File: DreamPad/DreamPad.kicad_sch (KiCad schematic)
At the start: 25 parts, among them J1 OLED Display, SW1 SW_Push, SW10 SW_Push, SW11 SW_Push, SW13 RotaryEncoder_Switch, SW2 SW_Push, SW3 SW_Push, SW5 SW_Push, SW6 SW_Push, SW7 SW_Push, SW9 SW_Push, U1 MOUDLE-SEEEDUINO-XIAO

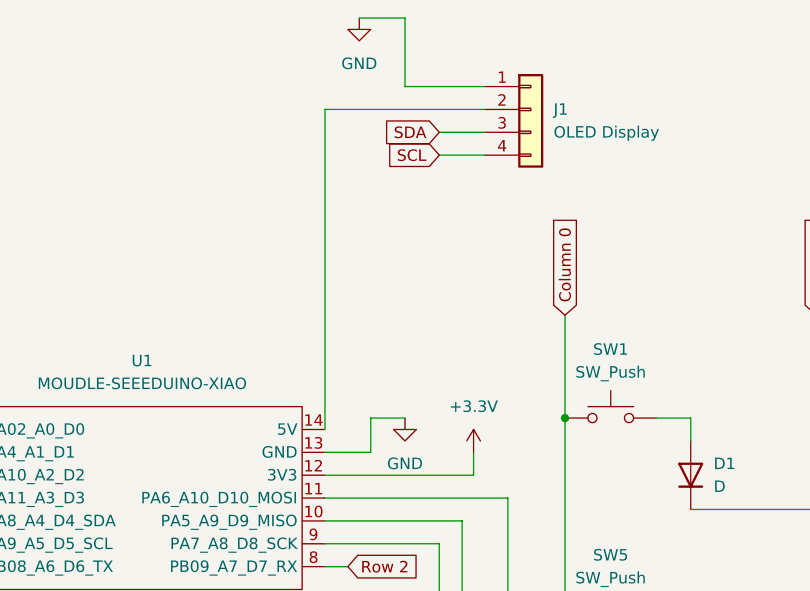
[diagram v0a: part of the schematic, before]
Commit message: Finalization and Readme
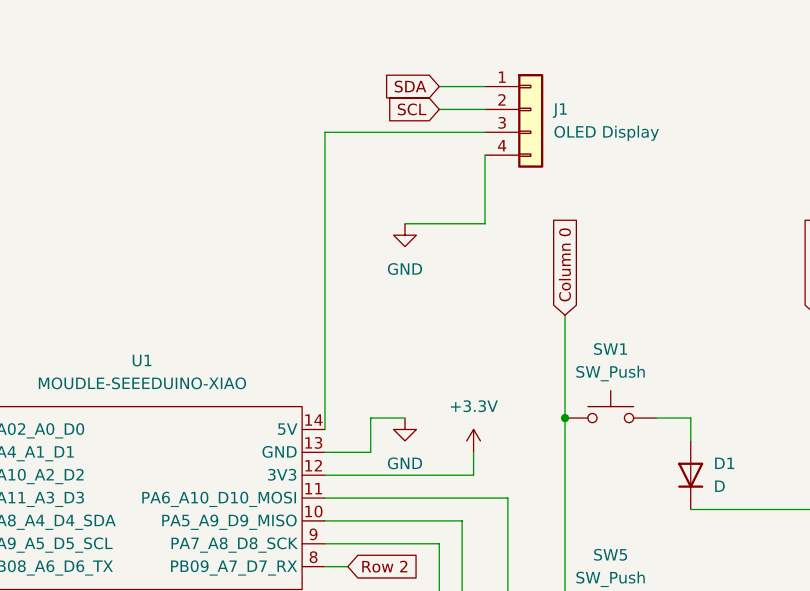
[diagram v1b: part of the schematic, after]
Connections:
- net GND: now also J1.4 (Pin_4); no longer J1.1 (Pin_1)
- net SCL: now also J1.2 (Pin_2); no longer J1.4 (Pin_4)
- net SDA: now also J1.1 (Pin_1); no longer J1.3 (Pin_3)
- net at U1.14 (5V): now also J1.3 (Pin_3); no longer J1.2 (Pin_2)
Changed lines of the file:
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@@
+	(wire
+		(pts
+			(xy 156.21 41.91) (xy 156.21 34.29)
+		)
+		(stroke
+			(width 0)
+			(type default)
+		)
+	)
 	(wire
 		(pts
@@
 	(wire
 		(pts
-			(xy 151.13 34.29) (xy 156.21 34.29)
-		)
-		(stroke
-			(width 0)
-			(type default)
-		)
-	)
-	(wire
-		(pts
-			(xy 142.24 19.05) (xy 147.32 19.05)
+			(xy 138.43 64.77) (xy 138.43 31.75)
 		)
 		(stroke
@@
 	(wire
 		(pts
-			(xy 138.43 29.21) (xy 138.43 64.77)
-		)
-		(stroke
-			(width 0)
-			(type default)
-		)
-	)
-	(wire
-		(pts
 			(xy 179.07 109.22) (xy 179.07 111.76)
 		)
@@
 	(wire
 		(pts
-			(xy 156.21 26.67) (xy 147.32 26.67)
-		)
-		(stroke
-			(width 0)
-			(type default)
-		)
-	)
-	(wire
-		(pts
 			(xy 88.9 69.85) (xy 97.79 69.85)
 		)
@@
 	(wire
 		(pts
+			(xy 151.13 29.21) (xy 156.21 29.21)
+		)
+		(stroke
+			(width 0)
+			(type default)
+		)
+	)
+	(wire
+		(pts
 			(xy 92.71 77.47) (xy 97.79 77.47)
 		)
@@
 	(wire
 		(pts
+			(xy 151.13 26.67) (xy 156.21 26.67)
+		)
+		(stroke
+			(width 0)
+			(type default)
+		)
+	)
+	(wire
+		(pts
 			(xy 232.41 63.5) (xy 232.41 66.04)
 		)
@@
 	(wire
 		(pts
-			(xy 151.13 31.75) (xy 156.21 31.75)
-		)
-		(stroke
-			(width 0)
-			(type default)
-		)
-	)
-	(wire
-		(pts
 			(xy 228.6 109.22) (xy 232.41 109.22)
 		)
@@
 	(wire
 		(pts
-			(xy 138.43 29.21) (xy 156.21 29.21)
-		)
-		(stroke
-			(width 0)
-			(type default)
-		)
-	)
-	(wire
-		(pts
 			(xy 128.27 97.79) (xy 121.92 97.79)
 		)
@@
 	(wire
 		(pts
-			(xy 147.32 19.05) (xy 147.32 26.67)
-		)
-		(stroke
-			(width 0)
-			(type default)
-		)
-	)
-	(wire
-		(pts
 			(xy 91.44 74.93) (xy 97.79 74.93)
 		)
@@
 	(wire
 		(pts
+			(xy 138.43 31.75) (xy 156.21 31.75)
+		)
+		(stroke
+			(width 0)
+			(type default)
+		)
+	)
+	(wire
+		(pts
 			(xy 91.44 72.39) (xy 97.79 72.39)
 		)
@@
 		(pts
 			(xy 95.25 82.55) (xy 95.25 80.01)
+		)
+		(stroke
+			(width 0)
+			(type default)
+		)
+	)
+	(wire
+		(pts
+			(xy 147.32 41.91) (xy 156.21 41.91)
 		)
 		(stroke
@@
 		)
 	)
+	(global_label "SCL"
+		(shape input)
+		(at 151.13 29.21 180)
+		(fields_autoplaced yes)
+		(effects
+			(font
+				(size 1.27 1.27)
+			)
+			(justify right)
+		)
+		(property "Intersheetrefs" "${INTERSHEET_REFS}"
+			(at 144.6372 29.21 0)
+			(hide yes)
+			(show_name no)
+			(do_not_autoplace no)
+			(effects
+				(font
+					(size 1.27 1.27)
+				)
+				(justify right)
+			)
+		)
+	)
 	(global_label "Row 2"
 		(shape input)
@@
 		)
 	)
+	(global_label "SDA"
+		(shape input)
+		(at 151.13 26.67 180)
+		(fields_autoplaced yes)
+		(effects
+			(font
+				(size 1.27 1.27)
+			)
+			(justify right)
+		)
+		(property "Intersheetrefs" "${INTERSHEET_REFS}"
+			(at 144.5767 26.67 0)
+			(hide yes)
+			(show_name no)
+			(do_not_autoplace no)
+			(effects
+				(font
+					(size 1.27 1.27)
+				)
+				(justify right)
+			)
+		)
+	)
 	(global_label "Row 1"
 		(shape input)
@@
 				)
 				(justify left)
-			)
-		)
-	)
-	(global_label "SDA"
-		(shape input)
-		(at 151.13 31.75 180)
-		(fields_autoplaced yes)
-		(effects
-			(font
-				(size 1.27 1.27)
-			)
-			(justify right)
-		)
-		(property "Intersheetrefs" "${INTERSHEET_REFS}"
-			(at 144.5767 31.75 0)
-			(hide yes)
-			(show_name no)
-			(do_not_autoplace no)
-			(effects
-				(font
-					(size 1.27 1.27)
-				)
-				(justify right)
-			)
-		)
-	)
-	(global_label "SCL"
-		(shape input)
-		(at 151.13 34.29 180)
-		(fields_autoplaced yes)
-		(effects
-			(font
-				(size 1.27 1.27)
-			)
-			(justify right)
-		)
-		(property "Intersheetrefs" "${INTERSHEET_REFS}"
-			(at 144.6372 34.29 0)
-			(hide yes)
-			(show_name no)
-			(do_not_autoplace no)
-			(effects
-				(font
-					(size 1.27 1.27)
-				)
-				(justify right)
 			)
 		)
@@
 	)
 	(symbol
-		(lib_id "power:GND")
-		(at 142.24 19.05 0)
-		(unit 1)
-		(body_style 1)
-		(exclude_from_sim no)
-		(in_bom yes)
-		(on_board yes)
-		(in_pos_files yes)
-		(dnp no)
-		(fields_autoplaced yes)
-		(property "Reference" "#PWR02"
-			(at 142.24 25.4 0)
-			(hide yes)
-			(show_name no)
-			(do_not_autoplace no)
-			(effects
-				(font
-					(size 1.27 1.27)
-				)
-			)
-		)
-		(property "Value" "GND"
-			(at 142.24 24.13 0)
-			(show_name no)
-			(do_not_autoplace no)
-			(effects
-				(font
-					(size 1.27 1.27)
-				)
-			)
-		)
-		(property "Footprint" ""
-			(at 142.24 19.05 0)
-			(hide yes)
-			(show_name no)
-			(do_not_autoplace no)
-			(effects
-				(font
-					(size 1.27 1.27)
-				)
-			)
-		)
-		(property "Datasheet" ""
-			(at 142.24 19.05 0)
-			(hide yes)
-			(show_name no)
-			(do_not_autoplace no)
-			(effects
-				(font
-					(size 1.27 1.27)
-				)
-			)
-		)
-		(property "Description" "Power symbol creates a global label with name \"GND\" , ground"
-			(at 142.24 19.05 0)
-			(hide yes)
-			(show_name no)
-			(do_not_autoplace no)
-			(effects
-				(font
-					(size 1.27 1.27)
-				)
-			)
-		)
-		(pin "1"
-		)
-		(instances
-			(project "DreamPad"
-				(path "/5ce19b80-1592-49cf-b0bb-42a567d40ee9"
-					(reference "#PWR02")
-					(unit 1)
-				)
-			)
-		)
-	)
-	(symbol
 		(lib_id "Mechanical:MountingHole")
 		(at 72.39 39.37 0)
@@
 					(unit 1)
 				)
+			)
+		)
+	)
+	(symbol
+		(lib_id "power:GND")
+		(at 147.32 41.91 0)
+		(unit 1)
+		(body_style 1)
+		(exclude_from_sim no)
+		(in_bom yes)
+		(on_board yes)
+		(in_pos_files yes)
+		(dnp no)
+		(fields_autoplaced yes)
+		(property "Reference" "#PWR02"
+			(at 147.32 48.26 0)
+			(hide yes)
+			(show_name no)
+			(do_not_autoplace no)
+			(effects
+				(font
+					(size 1.27 1.27)
+				)
+			)
+		)
+		(property "Value" "GND"
+			(at 147.32 46.99 0)
+			(show_name no)
+			(do_not_autoplace no)
+			(effects
+				(font
+					(size 1.27 1.27)
+				)
+			)
+		)
+		(property "Footprint" ""
+			(at 147.32 41.91 0)
+			(hide yes)
+			(show_name no)
+			(do_not_autoplace no)
+			(effects
+				(font
+					(size 1.27 1.27)
+				)
+			)
+		)
+		(property "Datasheet" ""
+			(at 147.32 41.91 0)
+			(hide yes)
+			(show_name no)
+			(do_not_autoplace no)
+			(effects
+				(font
+					(size 1.27 1.27)
+				)
+			)
+		)
+		(property "Description" "Power symbol creates a global label with name \"GND\" , ground"
+			(at 147.32 41.91 0)
+			(hide yes)
+			(show_name no)
+			(do_not_autoplace no)
+			(effects
+				(font
+					(size 1.27 1.27)
+				)
+			)
+		)
+		(pin "1"
+		)
+		(instances
+			(project "DreamPad"
+				(path "/5ce19b80-1592-49cf-b0bb-42a567d40ee9"
+					(reference "#PWR02")
+					(unit 1)
+				)
